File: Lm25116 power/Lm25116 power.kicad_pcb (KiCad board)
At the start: 2 copper layers, 43 parts, among them U1 SI7850ADP-T1-GE3, U2 SI7850ADP-T1-GE3, U3 LM25116MH

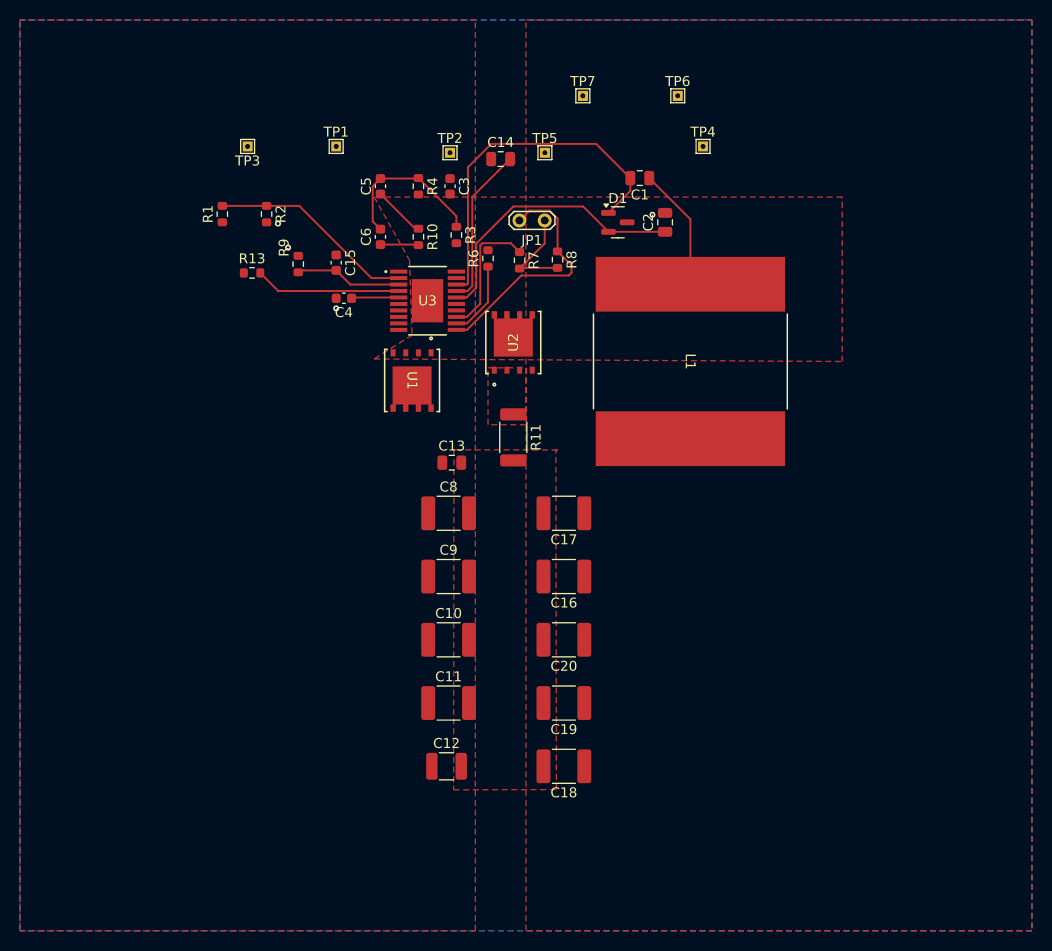
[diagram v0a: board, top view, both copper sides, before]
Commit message: New board test
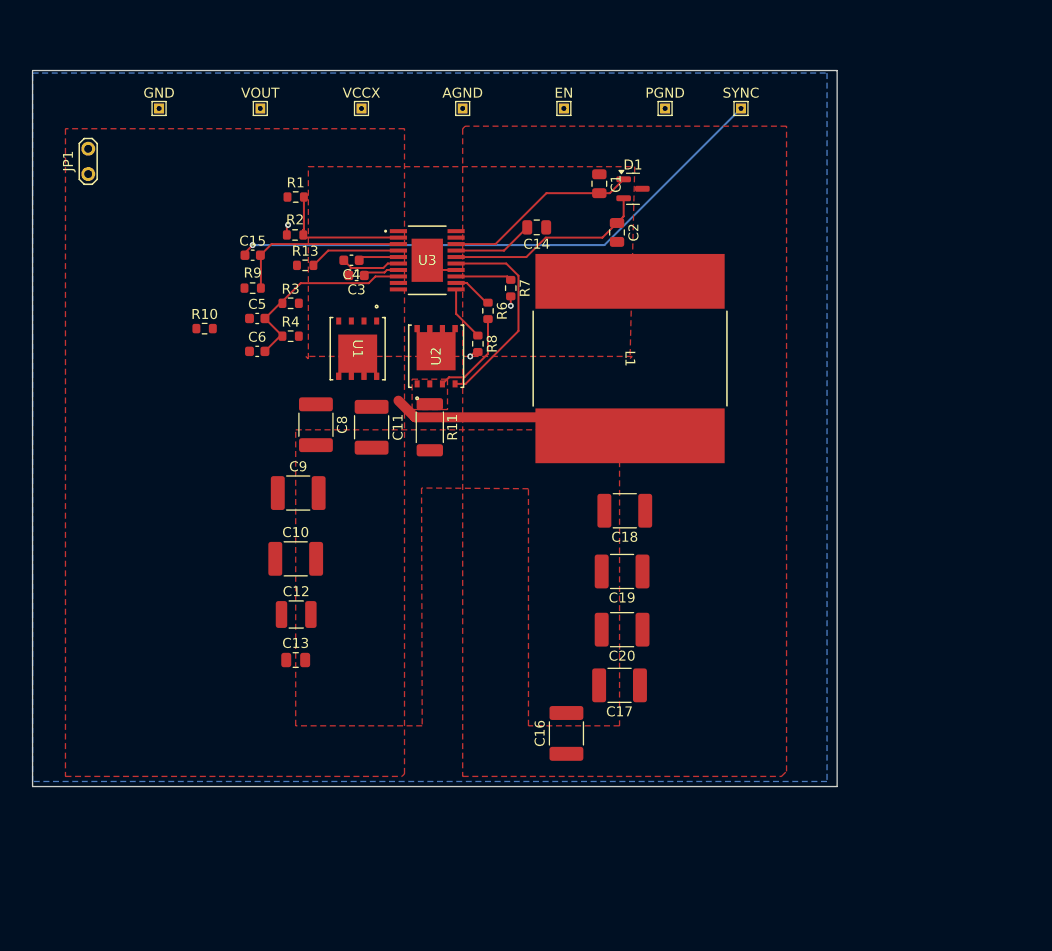
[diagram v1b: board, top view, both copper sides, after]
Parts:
- moved JP1 46.1 mm to (132.6, 62.5), turned to 90 degrees
- moved TP7 42.6 mm to (139.7, 55.9), turned to 180 degrees
- moved TP6 41.9 mm to (149.9, 55.9), turned to 180 degrees
- moved TP1 40.8 mm to (198.1, 55.9), turned to 180 degrees
- moved TP3 32.0 mm to (180.3, 55.9)
- moved C11 28.7 mm to (161.0, 87.9), turned to -90 degrees
- moved C18 26.4 mm to (186.5, 96.3)
- moved C13 25.3 mm to (153.4, 111.3)
- moved TP4 24.4 mm to (170.2, 55.9), turned to 180 degrees
- moved R10 23.4 mm to (144.3, 78.0), turned to 0 degrees
- moved TP2 22.0 mm to (190.5, 55.9), turned to 180 degrees
- moved C12 21.5 mm to (153.5, 106.7)
- moved R4 19.8 mm to (152.9, 78.7), turned to 0 degrees
- moved TP5 18.9 mm to (160.0, 55.9), turned to 180 degrees
- moved C17 18.2 mm to (185.9, 113.8)
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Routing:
- net Net-(C15-Pad1): track 0.00 -> 56.0 mm, vias 0 -> 1
- net +5V: track 0.00 -> 25.0 mm
- net Net-(U2-G): track 0.00 -> 20.9 mm
- net Net-(JP1-B): track 24.5 -> 5.54 mm
- net Net-(D1-K): track 36.0 -> 19.5 mm
- net Net-(U3-SW): track 12.4 -> 0.00 mm
- net Net-(R11-Pad1): track 0.00 -> 9.30 mm
- net Net-(D1-A): track 28.4 -> 20.3 mm
- net Net-(U3-VCCX): track 16.1 -> 8.11 mm
- net Net-(U3-CSG): track 13.2 -> 5.63 mm
- net Net-(D2-A): track 20.7 -> 13.5 mm
- net Net-(U3-RT/SYNC): track 10.5 -> 17.6 mm
- net Net-(U3-EN): track 14.6 -> 9.15 mm
- net Net-(U3-COMP): track 5.25 -> 0.00 mm
- net Net-(U3-FB): track 16.0 -> 20.2 mm
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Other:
- board outline added: 80.8 x 71.9 mm
